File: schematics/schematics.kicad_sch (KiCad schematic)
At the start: 32 parts, among them J1 USB_C_Receptacle_USB2.0_14P, J2 BAT, SW1 MS1, SW2 MS2, SW3 MS3, SW4 RST, SW5 BOOT, U1 ESP32-C3-WROOM-02, U2 MPU-6050, U3 AMS1117-3.3, U4 LTC4054ES5-4.2

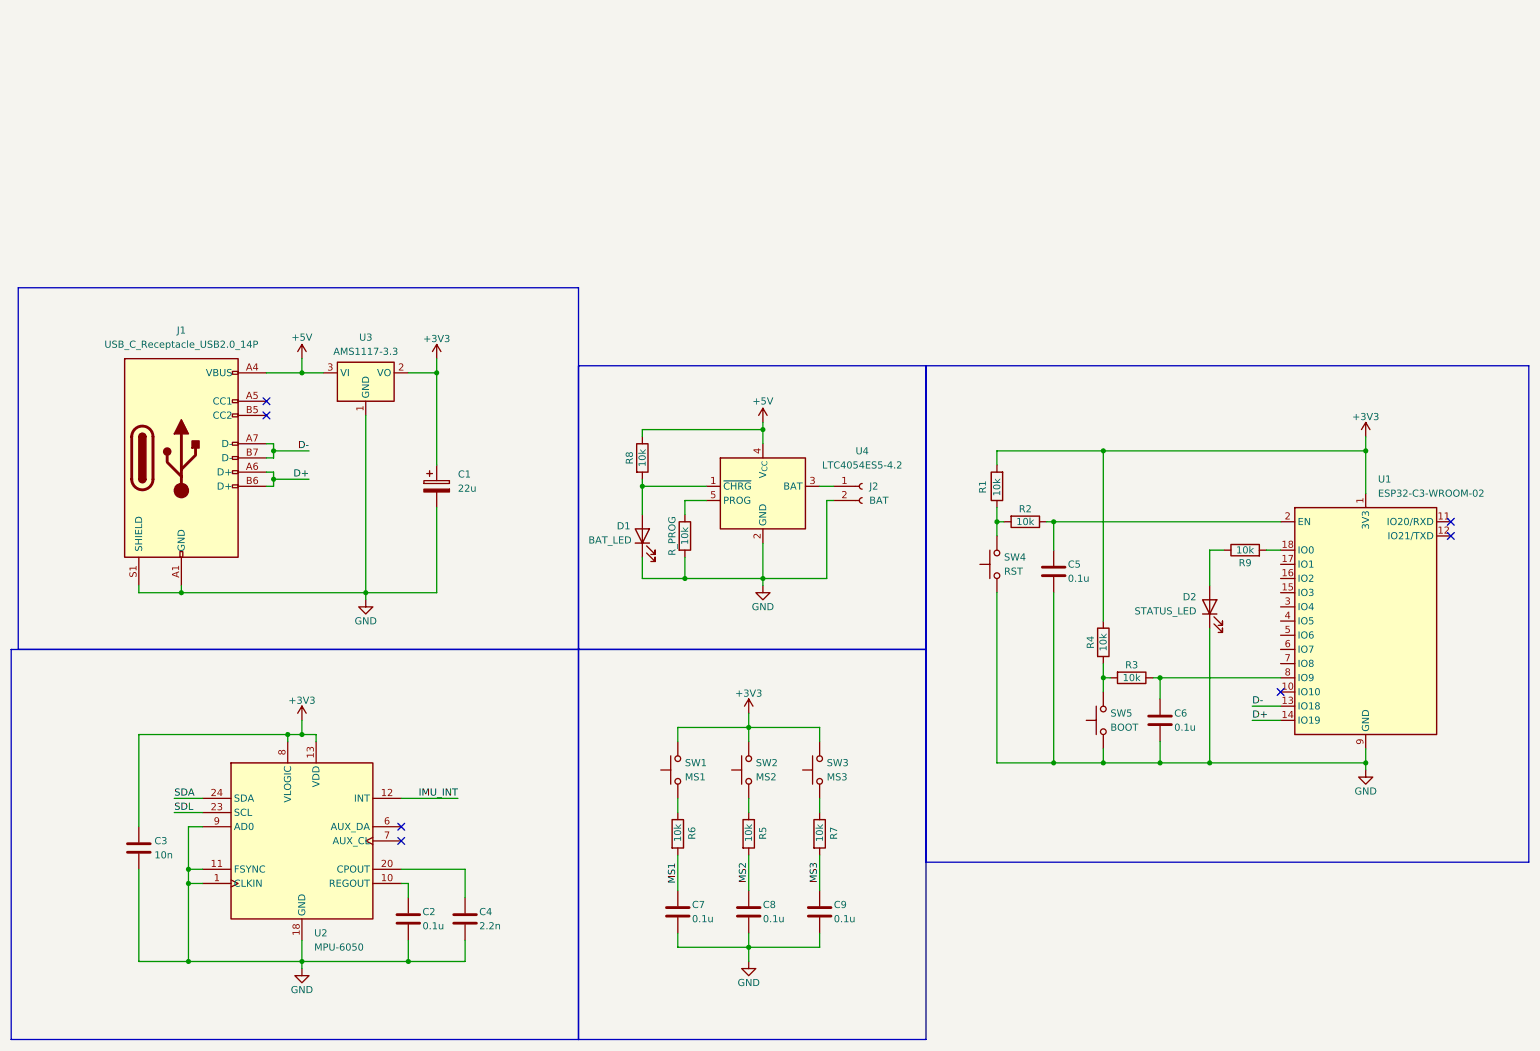
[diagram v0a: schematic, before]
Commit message: initial electronics
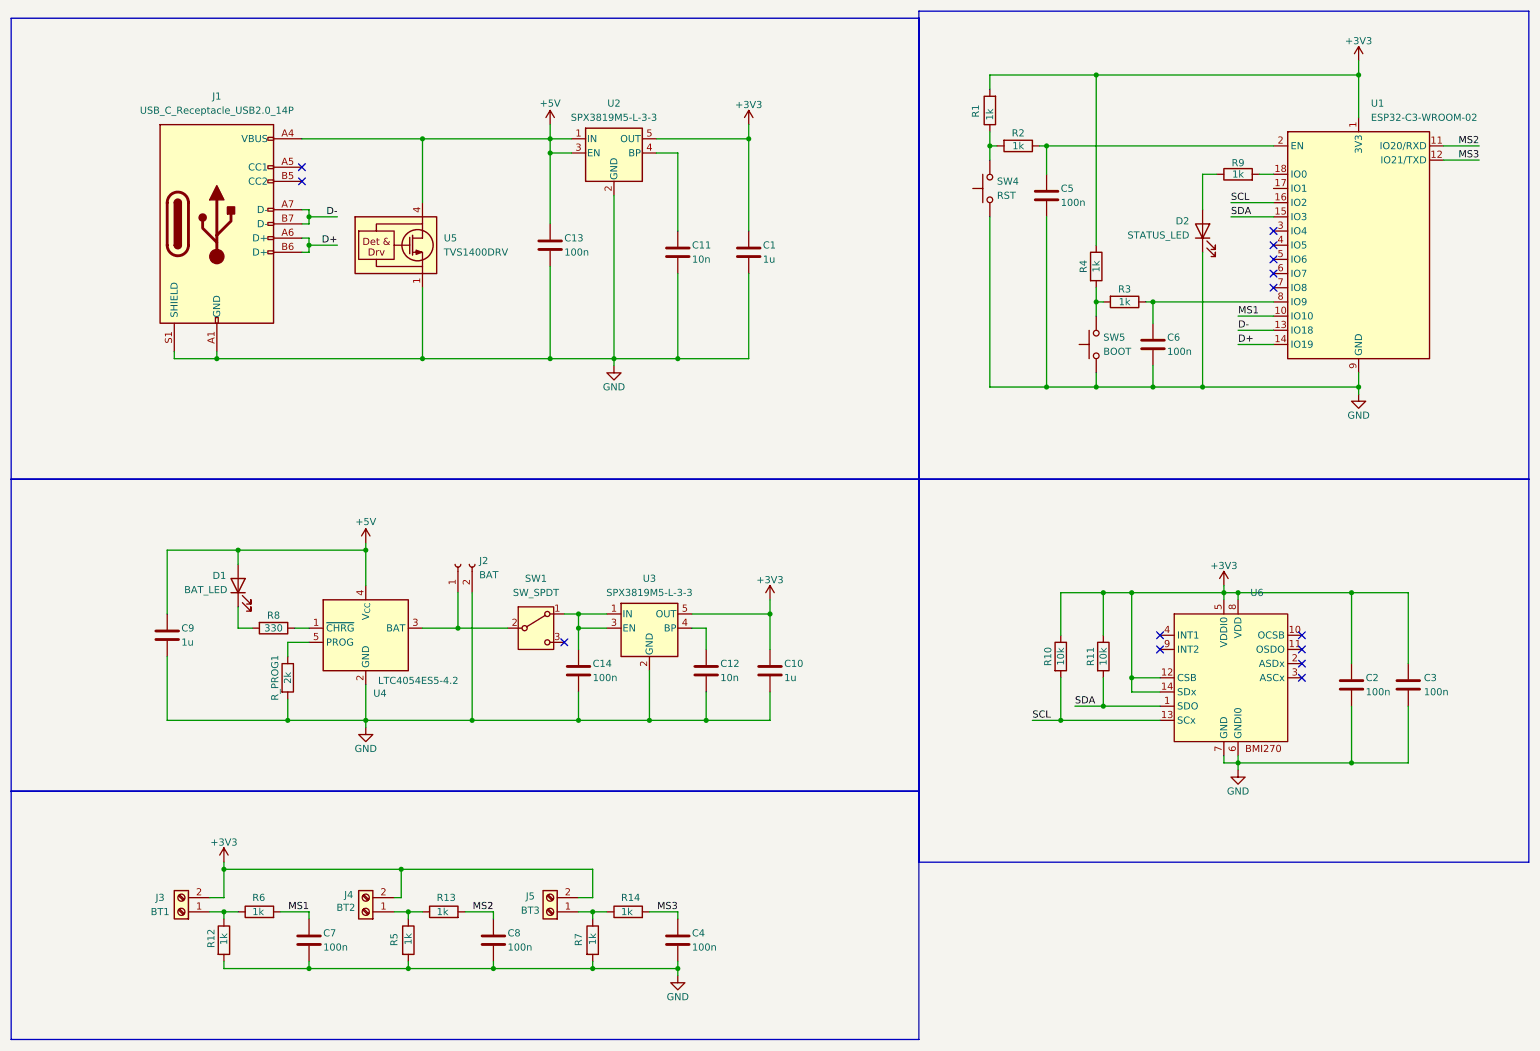
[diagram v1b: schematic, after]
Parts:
- removed C1: 22u, symbol Device:C_Polarized
- removed SW1: MS1, symbol Switch:SW_Push
- removed SW2: MS2, symbol Switch:SW_Push
- removed SW3: MS3, symbol Switch:SW_Push
- removed U2: MPU-6050, Sensor_Motion:InvenSense_QFN-24_4x4mm_P0.5mm, symbol Sensor_Motion:MPU-6050
- removed U3: AMS1117-3.3, Package_TO_SOT_SMD:SOT-223-3_TabPin2, symbol Regulator_Linear:AMS1117-3.3
- added C1, C10: 1u, Capacitor_SMD:C_0805_2012Metric, symbol Device:C
- added C11, C12: 10n, Capacitor_SMD:C_0603_1608Metric, symbol Device:C
- added C13, C14: 100n, Capacitor_SMD:C_0603_1608Metric, symbol Device:C
- added J3: BT1, TerminalBlock_Phoenix:TerminalBlock_Phoenix_MPT-0,5-2-2.54_1x02_P2.54mm_Horizontal, symbol Connector:Screw_Terminal_01x02
- added J4: BT2, TerminalBlock_Phoenix:TerminalBlock_Phoenix_MPT-0,5-2-2.54_1x02_P2.54mm_Horizontal, symbol Connector:Screw_Terminal_01x02
- added J5: BT3, TerminalBlock_Phoenix:TerminalBlock_Phoenix_MPT-0,5-2-2.54_1x02_P2.54mm_Horizontal, symbol Connector:Screw_Terminal_01x02
- added R10, R11: 10k, Resistor_SMD:R_0603_1608Metric, symbol Device:R
- added R12, R13, R14: 1k, Resistor_SMD:R_0603_1608Metric, symbol Device:R
- added SW1: SW_SPDT, Button_Switch_SMD:SW_SPDT_PCM12, symbol Switch:SW_SPDT
- added U2, U3: SPX3819M5-L-3-3, Package_TO_SOT_SMD:SOT-23-5, symbol Regulator_Linear:SPX3819M5-L-3-3
- added U5: TVS1400DRV, Package_SON:WSON-6-1EP_2x2mm_P0.65mm_EP1x1.6mm, symbol Power_Protection:TVS1400DRV
- added U6: ~, Package_LGA:Bosch_LGA-14_3x2.5mm_P0.5mm, symbol BMI270:BMI270
- C2, C5, C6, C7, C8: value 0.1u -> 100n; footprint (none) -> Capacitor_SMD:C_0603_1608Metric
- C3: value 10n -> 100n; footprint (none) -> Capacitor_SMD:C_0603_1608Metric
- C4: value 2.2n -> 100n; footprint (none) -> Capacitor_SMD:C_0603_1608Metric
- C9: value 0.1u -> 1u; footprint (none) -> Capacitor_SMD:C_0805_2012Metric
- D1, D2: footprint (none) -> LED_THT:LED_D1.8mm_W1.8mm_H2.4mm_Horizontal_O1.27mm_Z1.6mm
- J1: footprint (none) -> Connector_USB:USB_C_Receptacle_GCT_USB4110
- J2: footprint (none) -> Connector_JST:JST_PH_B2B-PH-K_1x02_P2.00mm_Vertical
- R1, R2, R3, R4, R5, R6, R7, R9: value 10k -> 1k; footprint (none) -> Resistor_SMD:R_0603_1608Metric
- R8: value 10k -> 330; footprint (none) -> Resistor_SMD:R_0603_1608Metric
- R_PROG1: renamed from R_PROG; value 10k -> 2k; footprint (none) -> Resistor_SMD:R_0603_1608Metric
- SW4, SW5: footprint (none) -> Button_Switch_SMD:SW_Push_1P1T_NO_CK_KMR2
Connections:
- net +3V3: now also C2.1, C1.1, C10.1, J3.2 (Pin_2), J4.2 (Pin_2), J5.2 (Pin_2), R10.1, R11.1, U2.5 (OUT), U3.5 (OUT), U6.12 (CSB), U6.14 (SDx), U6.5 (VDDI0), U6.8 (VDD)
- net +5V: now also C9.1, D1.2 (A), C13.1, U2.1 (IN), U2.3 (EN), U5.4 (IN), U5.5 (IN), U5.6 (IN); no longer R8.1
- net GND: now also R5.2, R7.2, C1.2, C10.2, C11.2, C12.2, C13.2, C14.2, R12.2, U2.2 (GND), U3.2 (GND), U5.1 (GND), U5.2 (GND), U5.3 (GND), U5.7 (GND), U6.6 (GNDI0), U6.7 (GND); no longer D1.1 (K)
- net MS1: now also U1.10 (IO10)
- net MS2: now also U1.11 (IO20/RXD), R13.2; no longer R5.2
- net MS3: now also C4.1, U1.12 (IO21/TXD), R14.2; no longer C9.1, R7.2
- net SDA: now also U1.15 (IO3), R11.2, U6.1 (SDO)
- net at R5.1: now also J4.1 (Pin_1), R13.1
- net at R6.1: now also J3.1 (Pin_1), R12.1
- net at J2.1 (Pin_1), U4.3 (BAT): now also SW1.2 (B)
- net at R7.1: now also J5.1 (Pin_1), R14.1
- net SCL: now reaches U1.16 (IO2)
- net SCL: now also R10.2, U6.13 (SCx)
- new net: C14.1, SW1.1 (A), U3.1 (IN), U3.3 (EN)
- new net: R8.1, U4.1 (~{CHRG})
- new net: C11.1, U2.4 (BP)
- new net: C12.1, U3.4 (BP)
- new net: D1.1 (K), R8.2
- no-connect marks 7 -> 14
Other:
- moved on the sheet: C2, C3, C5, C6, C7, C8, D1, D2, J1, J2, R1, R2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
